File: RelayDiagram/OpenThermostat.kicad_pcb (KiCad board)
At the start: 2 copper layers, 152.5 x 101.5 mm, 90 parts, among them J1 Conn_01x08_Female, J2 Conn_01x15_Female, J3 Conn_01x15_Female, J4 Conn_01x09_Female, Q1 Q_NMOS_DGS, Q10 Q_NMOS_DGS, Q11 Q_NMOS_DGS, Q12 Q_NMOS_DGS, Q2 Q_NMOS_DGS, Q3 Q_NMOS_DGS, Q4 Q_NMOS_DGS, Q5 Q_NMOS_DGS, Q6 Q_NMOS_DGS, Q7 Q_NMOS_DGS, Q8 Q_NMOS_DGS, Q9 Q_NMOS_DGS, SW2 SW_Push, SW3 SW_Push, SW4 SW_Push, SW5 SW_Push, SW6 SW_Push, U1 PCF8574, U10 MB10S-13, U11 L7805CV, U2 LCD, U3 DHT11, U4 EE2-3TNU-L_DPDT_Relay, U5 EE2-3TNU-L_DPDT_Relay, U6 EE2-3TNU-L_DPDT_Relay, U7 EE2-3TNU-L_DPDT_Relay, U8 EE2-3TNU-L_DPDT_Relay, U9 EE2-3TNU-L_DPDT_Relay

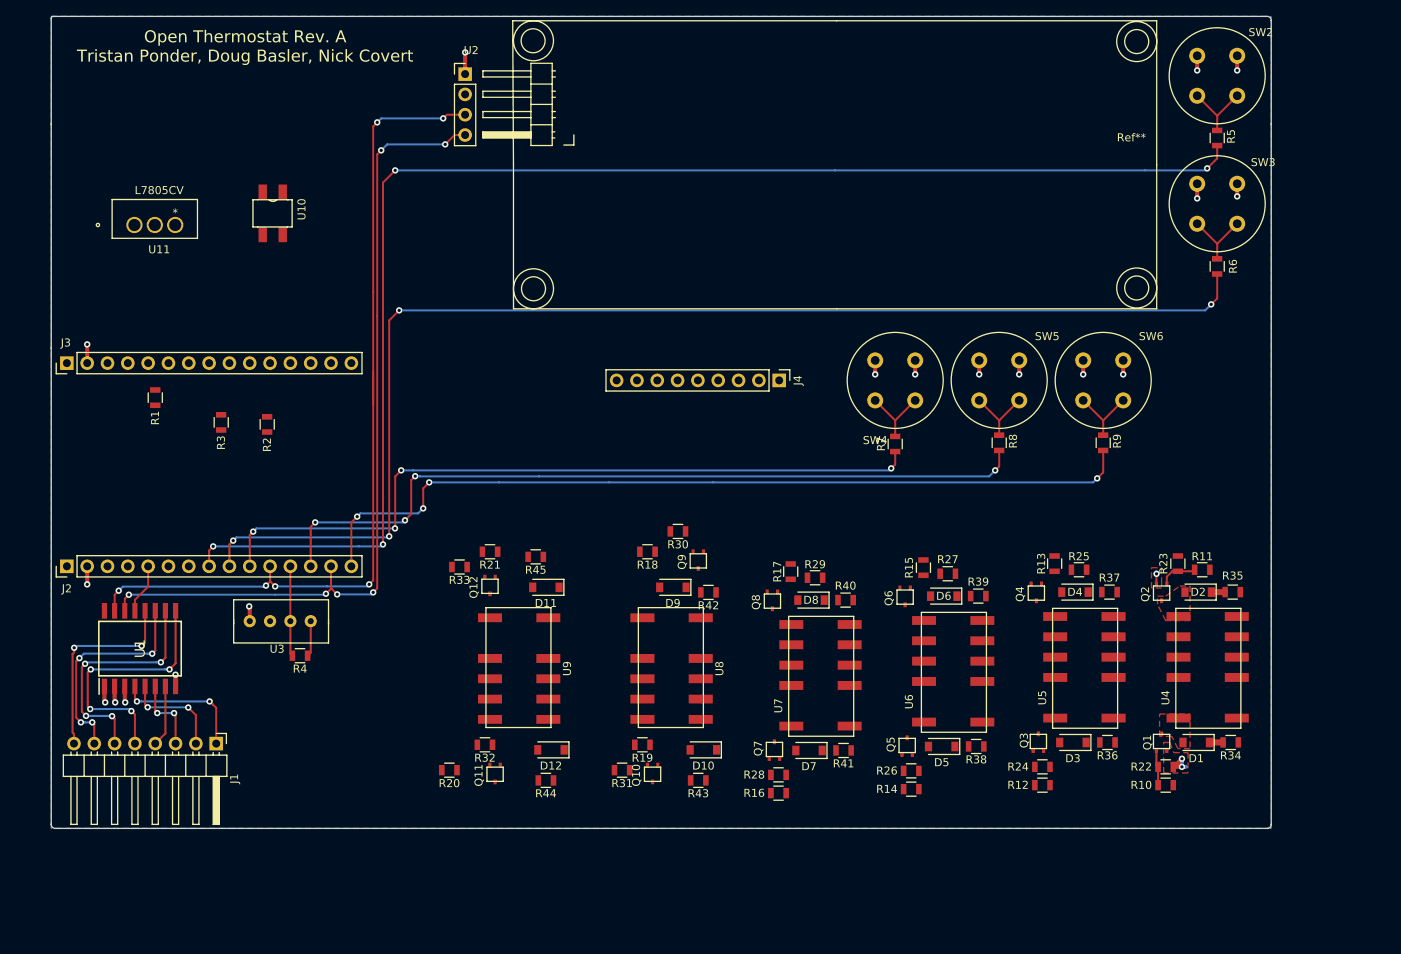
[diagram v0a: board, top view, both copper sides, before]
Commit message: Change
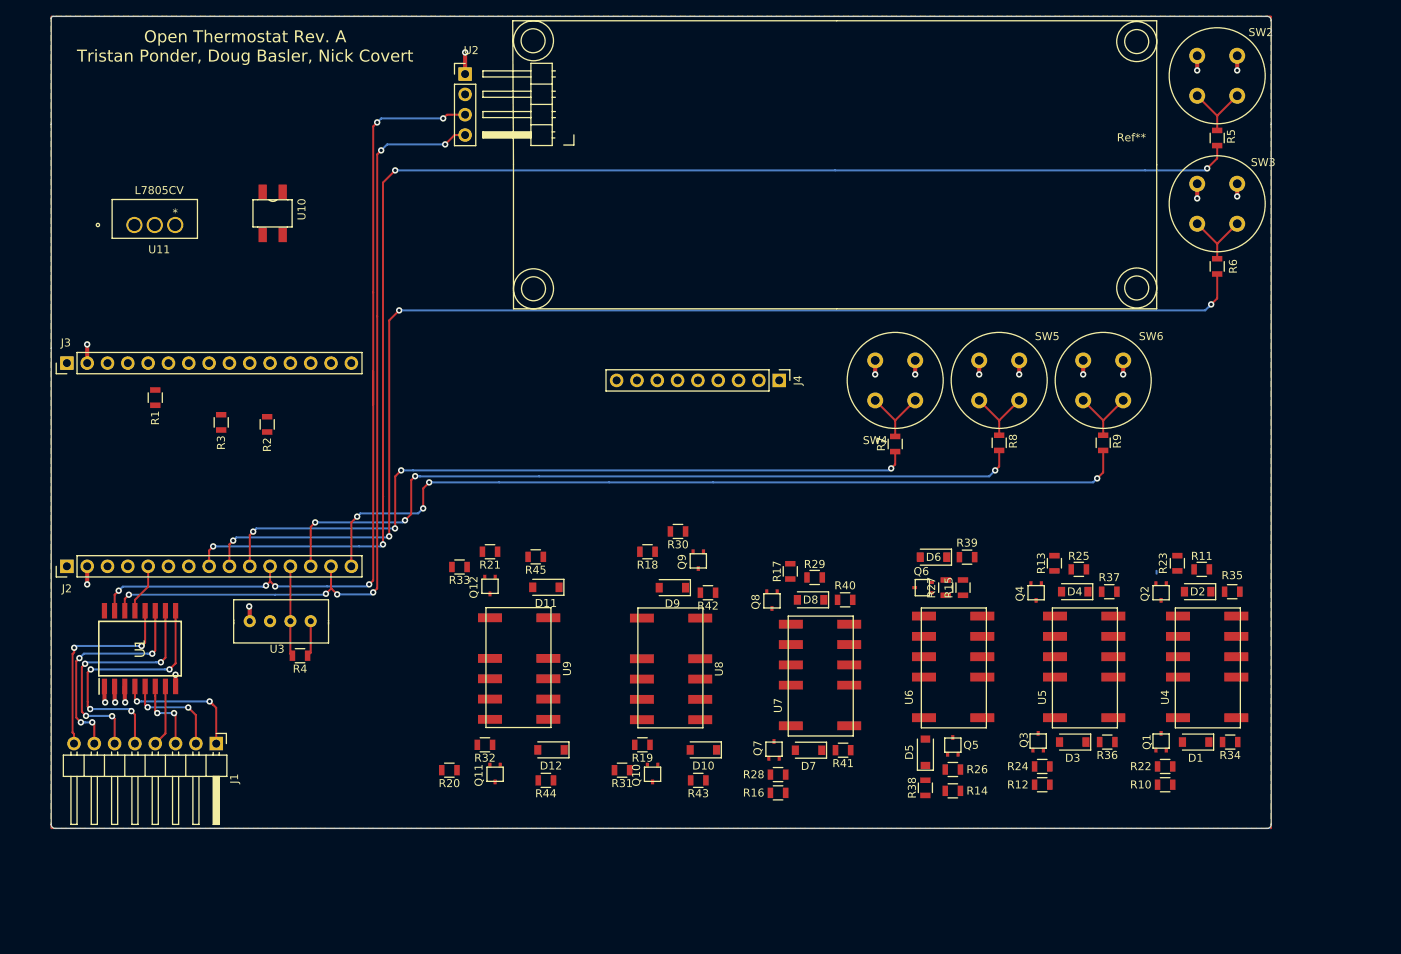
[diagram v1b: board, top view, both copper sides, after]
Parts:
- moved R38 8.19 mm to (160.3, 153.9), turned to 90 degrees
- moved Q5 5.71 mm to (163.7, 149.7)
- moved R15 5.54 mm to (165.0, 128.9)
- moved R14 5.20 mm to (163.7, 154.3)
- moved R26 5.20 mm to (163.7, 151.6)
- moved R39 5.07 mm to (165.5, 125.1)
- moved D6 5.03 mm to (161.3, 125.1)
- moved Q6 3.29 mm to (161.0, 128.9), turned to 90 degrees
- moved D5 2.16 mm to (160.3, 149.5), turned to 90 degrees
- moved R27 1.76 mm to (162.8, 128.9), turned to 90 degrees
- moved U6 0.55 mm to (167.4, 145.2)
- moved R35 0.08 mm to (198.6, 129.4)
- moved Q1 0.08 mm to (189.7, 149.2)
- moved Q2 0.08 mm to (189.7, 128.4)
- moved R11 0.08 mm to (194.8, 126.6)
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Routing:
- net GND: track 39.6 -> 34.7 mm, vias 21 -> 18
- net Net-(Q2-Pad2): track 4.75 -> 0.00 mm
- net Net-(Q1-Pad2): track 4.40 -> 0.00 mm
- net Net-(D2-Pad1): track 1.72 -> 0.00 mm
- net Net-(D1-Pad1): track 1.72 -> 0.00 mm
- added copper zone on F.Cu, net +5V
- removed copper zone on F.Cu, net GND
- removed copper zone on F.Cu, net Net-(D1-Pad2)
- removed copper zone on F.Cu, net Net-(D2-Pad2)

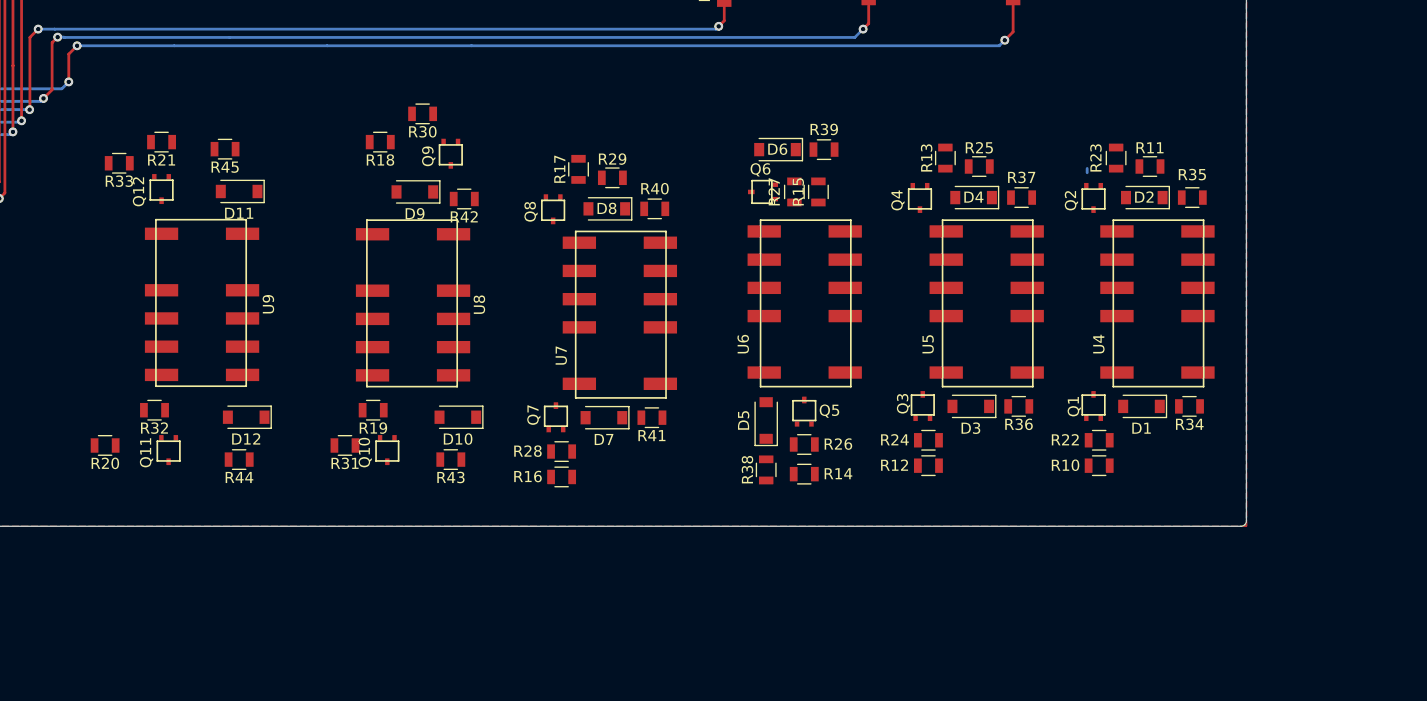
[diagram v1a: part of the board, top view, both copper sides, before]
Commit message: PCB updates
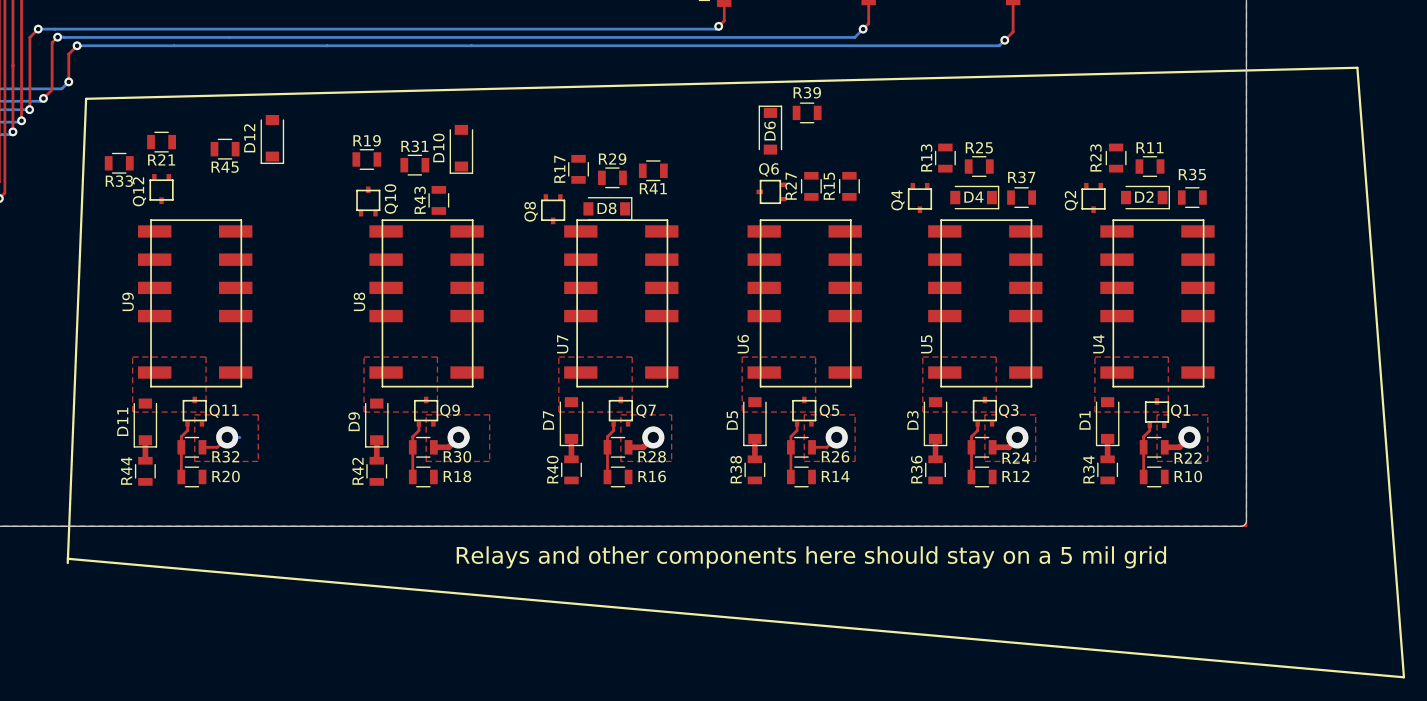
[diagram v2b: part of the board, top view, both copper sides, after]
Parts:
- moved R18 30.4 mm to (129.4, 154.6), turned to 0 degrees
- moved R30 30.0 mm to (129.4, 151.9), turned to 0 degrees
- moved R31 26.0 mm to (128.7, 126.5), turned to 0 degrees
- moved R42 25.7 mm to (125.2, 154.1), turned to 90 degrees
- moved Q9 25.4 mm to (129.7, 149.7), turned to 0 degrees
- moved D12 25.2 mm to (115.8, 124.1), turned to 90 degrees
- moved R40 24.7 mm to (142.7, 153.9), turned to 90 degrees
- moved D10 24.2 mm to (132.8, 125.0), turned to 90 degrees
- moved R43 23.4 mm to (130.8, 129.7), turned to 90 degrees
- moved R19 22.6 mm to (124.3, 126.0), turned to 0 degrees
- moved D11 22.4 mm to (104.4, 149.6), turned to 90 degrees
- moved R41 22.2 mm to (150.1, 127.0)
- moved D9 21.0 mm to (125.2, 149.6), turned to 90 degrees
- moved Q10 20.4 mm to (124.5, 130.8), turned to 0 degrees
- moved U8 15.1 mm to (133.3, 145.2), turned to 90 degrees
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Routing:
- net GND: track 34.7 -> 53.7 mm, vias 18 -> 24
- net Net-(Q9-Pad2): track 0.00 -> 5.06 mm
- net Net-(Q7-Pad2): track 0.00 -> 5.06 mm
- net Net-(Q5-Pad2): track 0.00 -> 5.06 mm
- net Net-(Q3-Pad2): track 0.00 -> 5.06 mm
- net Net-(Q11-Pad2): track 0.00 -> 5.06 mm
- net Net-(Q1-Pad2): track 0.00 -> 4.93 mm
- net Net-(D9-Pad1): track 0.00 -> 1.84 mm
- net Net-(D7-Pad1): track 0.00 -> 1.84 mm
- net Net-(D5-Pad1): track 0.00 -> 1.84 mm
- net Net-(D3-Pad1): track 0.00 -> 1.84 mm
- net Net-(D11-Pad1): track 0.00 -> 1.84 mm
- net Net-(D1-Pad1): track 0.00 -> 1.84 mm
- added copper zone on F.Cu, net GND
- added copper zone on F.Cu, net Net-(D1-Pad2)
- added copper zone on F.Cu, net Net-(D11-Pad2)
- added copper zone on F.Cu, net Net-(D3-Pad2)
- added copper zone on F.Cu, net Net-(D5-Pad2)
- added copper zone on F.Cu, net Net-(D7-Pad2)
- added copper zone on F.Cu, net Net-(D9-Pad2)
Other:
- board text added: "Relays and other components here should stay on a 5 mil grid"
